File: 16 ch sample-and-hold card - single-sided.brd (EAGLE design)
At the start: 66 x 32.1 mm, 85 parts, among them IC1 MAX306CWI, IC2 TL074D, IC3 TL074D, IC4 TL074D, IC5 TL074D

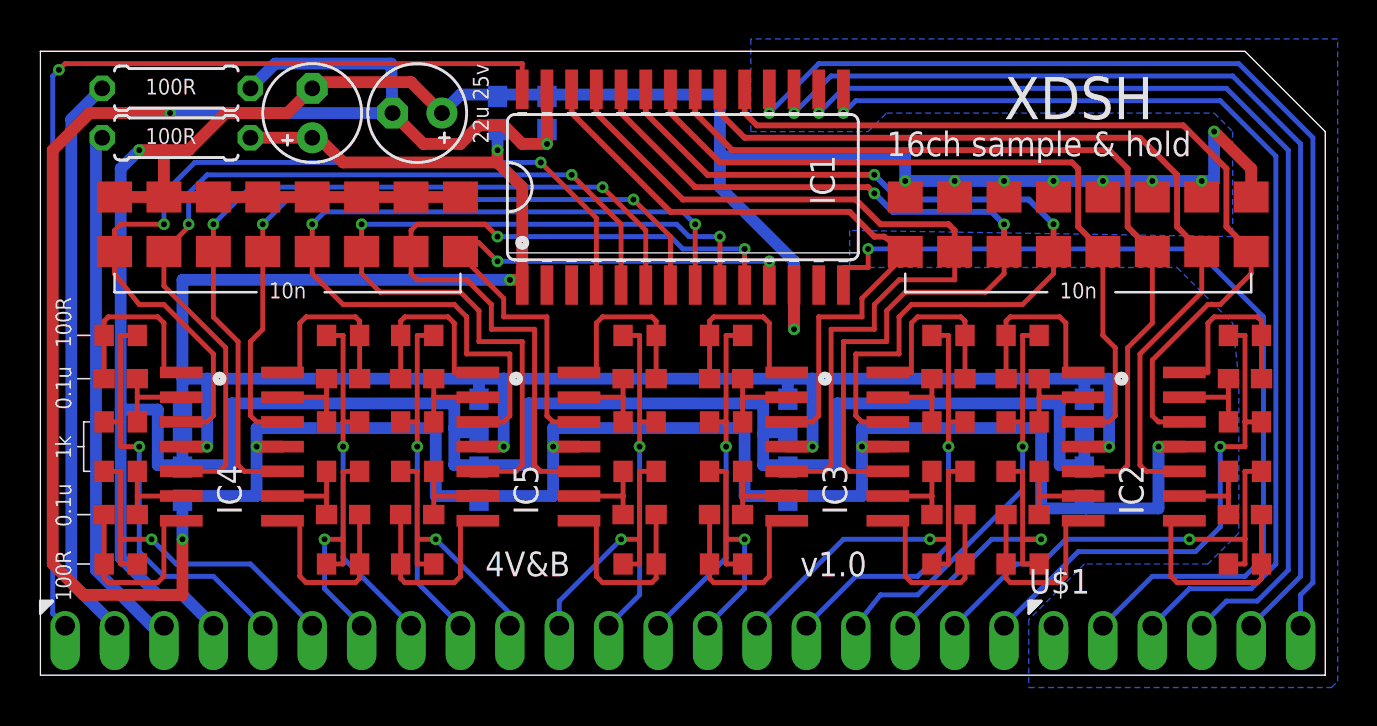
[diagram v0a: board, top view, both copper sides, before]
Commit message: Last commit before moving multiplexer to separate repo
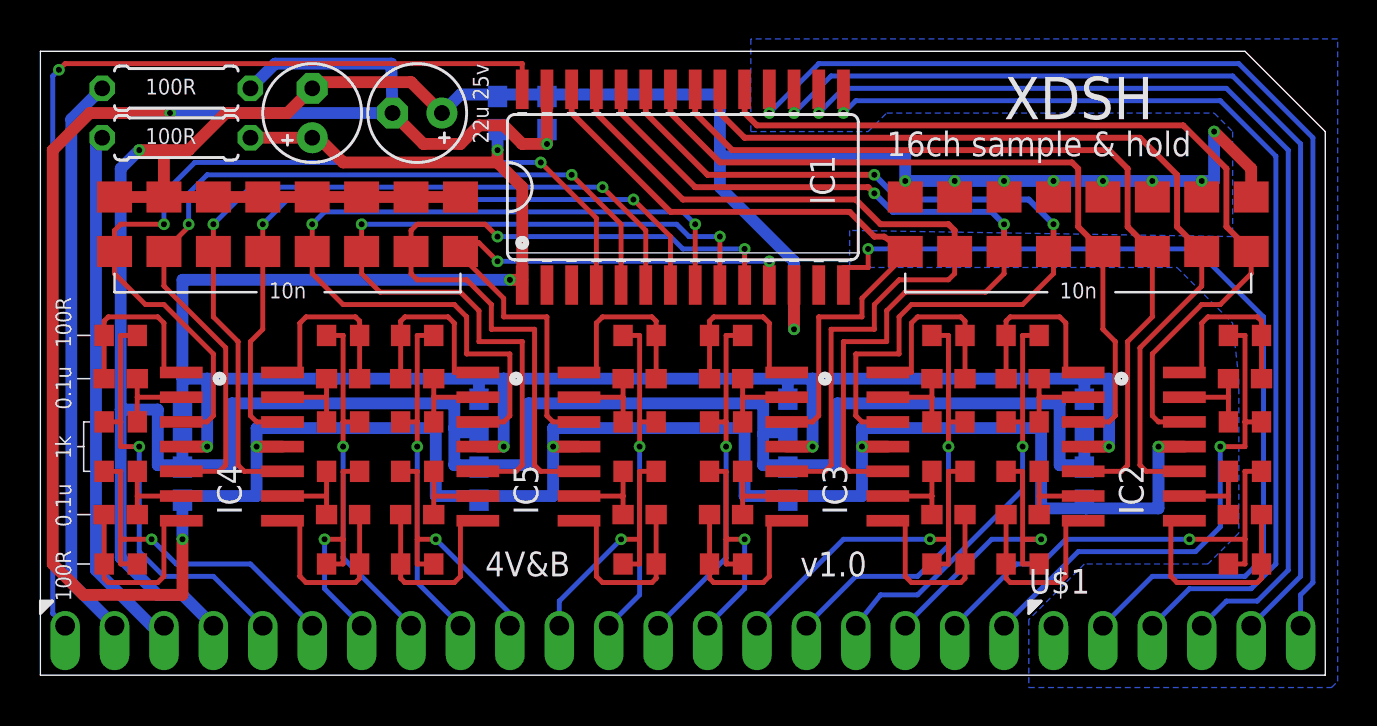
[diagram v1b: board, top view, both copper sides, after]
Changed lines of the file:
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@@
 <wire x1="58.7975" y1="13.0175" x2="57.4675" y2="13.0175" width="0.254" layer="1"/>
 <wire x1="57.4675" y1="13.0175" x2="57.15" y2="13.335" width="0.254" layer="1"/>
-<wire x1="57.15" y1="13.335" x2="57.15" y2="16.1925" width="0.254" layer="1"/>
-<wire x1="57.15" y1="16.1925" x2="60.0075" y2="19.05" width="0.254" layer="1"/>
-<wire x1="60.0075" y1="19.05" x2="60.6425" y2="19.05" width="0.254" layer="1"/>
+<wire x1="57.15" y1="13.335" x2="57.15" y2="16.51" width="0.254" layer="1"/>
+<wire x1="57.15" y1="16.51" x2="59.69" y2="19.05" width="0.254" layer="1"/>
+<wire x1="59.69" y1="19.05" x2="60.6425" y2="19.05" width="0.254" layer="1"/>
 <wire x1="60.6425" y1="19.05" x2="62.23" y2="20.6375" width="0.254" layer="1"/>
 <wire x1="62.23" y1="20.6375" x2="62.23" y2="21.7775" width="0.254" layer="1"/>
@@
 <wire x1="58.7975" y1="10.4775" x2="56.8325" y2="10.4775" width="0.254" layer="1"/>
 <wire x1="56.8325" y1="10.4775" x2="56.515" y2="10.795" width="0.254" layer="1"/>
-<wire x1="56.515" y1="10.795" x2="56.515" y2="16.51" width="0.254" layer="1"/>
-<wire x1="56.515" y1="16.51" x2="59.69" y2="19.685" width="0.254" layer="1"/>
-<wire x1="59.69" y1="19.685" x2="59.69" y2="21.7775" width="0.254" layer="1"/>
+<wire x1="56.515" y1="10.795" x2="56.515" y2="16.8275" width="0.254" layer="1"/>
+<wire x1="56.515" y1="16.8275" x2="59.69" y2="20.0025" width="0.254" layer="1"/>
+<wire x1="59.69" y1="20.0025" x2="59.69" y2="21.7775" width="0.254" layer="1"/>
 <wire x1="34.925" y1="30.1117" x2="34.925" y2="28.8925" width="0.3048" layer="1"/>
 <wire x1="34.925" y1="28.8925" x2="36.195" y2="27.6225" width="0.3048" layer="1"/>
@@
 <wire x1="53.5975" y1="10.4775" x2="55.5625" y2="10.4775" width="0.254" layer="1"/>
 <wire x1="55.5625" y1="10.4775" x2="55.88" y2="10.795" width="0.254" layer="1"/>
-<wire x1="55.88" y1="10.795" x2="55.88" y2="16.8275" width="0.254" layer="1"/>
-<wire x1="55.88" y1="16.8275" x2="57.15" y2="18.0975" width="0.254" layer="1"/>
-<wire x1="57.15" y1="18.0975" x2="57.15" y2="21.59" width="0.254" layer="1"/>
+<wire x1="55.88" y1="10.795" x2="55.88" y2="17.145" width="0.254" layer="1"/>
+<wire x1="55.88" y1="17.145" x2="57.15" y2="18.415" width="0.254" layer="1"/>
+<wire x1="57.15" y1="18.415" x2="57.15" y2="21.59" width="0.254" layer="1"/>
 <wire x1="57.15" y1="21.59" x2="57.3375" y2="21.7775" width="0.254" layer="1"/>
 <wire x1="57.3375" y1="21.7775" x2="57.15" y2="21.7775" width="0.254" layer="1"/>
@@
 <wire x1="53.5975" y1="13.0175" x2="54.9275" y2="13.0175" width="0.254" layer="1"/>
 <wire x1="54.9275" y1="13.0175" x2="55.245" y2="13.335" width="0.254" layer="1"/>
-<wire x1="55.245" y1="13.335" x2="55.245" y2="16.8275" width="0.254" layer="1"/>
-<wire x1="55.245" y1="16.8275" x2="54.61" y2="17.4625" width="0.254" layer="1"/>
-<wire x1="54.61" y1="17.4625" x2="54.61" y2="21.7775" width="0.254" layer="1"/>
+<wire x1="55.245" y1="13.335" x2="55.245" y2="17.145" width="0.254" layer="1"/>
+<wire x1="55.245" y1="17.145" x2="54.61" y2="17.78" width="0.254" layer="1"/>
+<wire x1="54.61" y1="17.78" x2="54.61" y2="21.7775" width="0.254" layer="1"/>
 <wire x1="32.385" y1="30.1117" x2="32.385" y2="28.8925" width="0.3048" layer="1"/>
 <wire x1="32.385" y1="28.8925" x2="34.925" y2="26.3525" width="0.3048" layer="1"/>
@@
 <contactref element="C14" pad="1"/>
 <wire x1="62.7625" y1="15.24" x2="62.7625" y2="17.4625" width="0.254" layer="1"/>
-<wire x1="58.7975" y1="15.5575" x2="60.0075" y2="15.5575" width="0.254" layer="1"/>
-<wire x1="60.0075" y1="15.5575" x2="60.0075" y2="18.0975" width="0.254" layer="1"/>
-<wire x1="60.0075" y1="18.0975" x2="60.325" y2="18.415" width="0.254" layer="1"/>
+<wire x1="58.7975" y1="15.5575" x2="59.69" y2="15.5575" width="0.254" layer="1"/>
+<wire x1="59.69" y1="15.5575" x2="59.69" y2="18.0975" width="0.254" layer="1"/>
+<wire x1="59.69" y1="18.0975" x2="60.0075" y2="18.415" width="0.254" layer="1"/>
 <wire x1="62.7625" y1="17.4625" x2="62.7625" y2="18.2" width="0.254" layer="1"/>
 <wire x1="62.7625" y1="18.2" x2="62.5475" y2="18.415" width="0.254" layer="1"/>
-<wire x1="62.5475" y1="18.415" x2="60.325" y2="18.415" width="0.254" layer="1"/>
+<wire x1="62.5475" y1="18.415" x2="60.0075" y2="18.415" width="0.254" layer="1"/>
 </signal>
 <signal name="N$7">
@@
 <wire x1="42.8625" y1="17.78" x2="42.8625" y2="19.05" width="0.254" layer="1"/>
 <wire x1="42.8625" y1="19.05" x2="44.1325" y2="20.32" width="0.254" layer="1"/>
-<wire x1="44.1325" y1="20.32" x2="46.99" y2="20.32" width="0.254" layer="1"/>
-<wire x1="46.99" y1="20.32" x2="46.99" y2="21.7775" width="0.254" layer="1"/>
+<wire x1="44.1325" y1="20.32" x2="46.6725" y2="20.32" width="0.254" layer="1"/>
+<wire x1="46.6725" y1="20.32" x2="46.99" y2="20.6375" width="0.254" layer="1"/>
+<wire x1="46.99" y1="20.6375" x2="46.99" y2="21.7775" width="0.254" layer="1"/>
 <wire x1="28.575" y1="30.1117" x2="28.575" y2="28.8925" width="0.3048" layer="1"/>
 <wire x1="28.575" y1="28.8925" x2="33.02" y2="24.4475" width="0.3048" layer="1"/>
@@
 <via x="25.7175" y="26.3525" extent="1-16" drill="0.3048"/>
 <wire x1="3.81" y1="21.7775" x2="3.81" y2="20.6375" width="0.254" layer="1"/>
-<wire x1="3.81" y1="20.6375" x2="5.08" y2="19.05" width="0.254" layer="1"/>
-<wire x1="5.08" y1="19.05" x2="6.35" y2="19.05" width="0.254" layer="1"/>
+<wire x1="3.81" y1="20.6375" x2="5.3975" y2="19.05" width="0.254" layer="1"/>
+<wire x1="5.3975" y1="19.05" x2="6.35" y2="19.05" width="0.254" layer="1"/>
 <wire x1="6.35" y1="19.05" x2="8.89" y2="16.51" width="0.254" layer="1"/>
 <wire x1="25.7175" y1="26.3525" x2="7.9375" y2="26.3525" width="0.254" layer="16"/>
